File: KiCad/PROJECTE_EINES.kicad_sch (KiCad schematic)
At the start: 5 parts

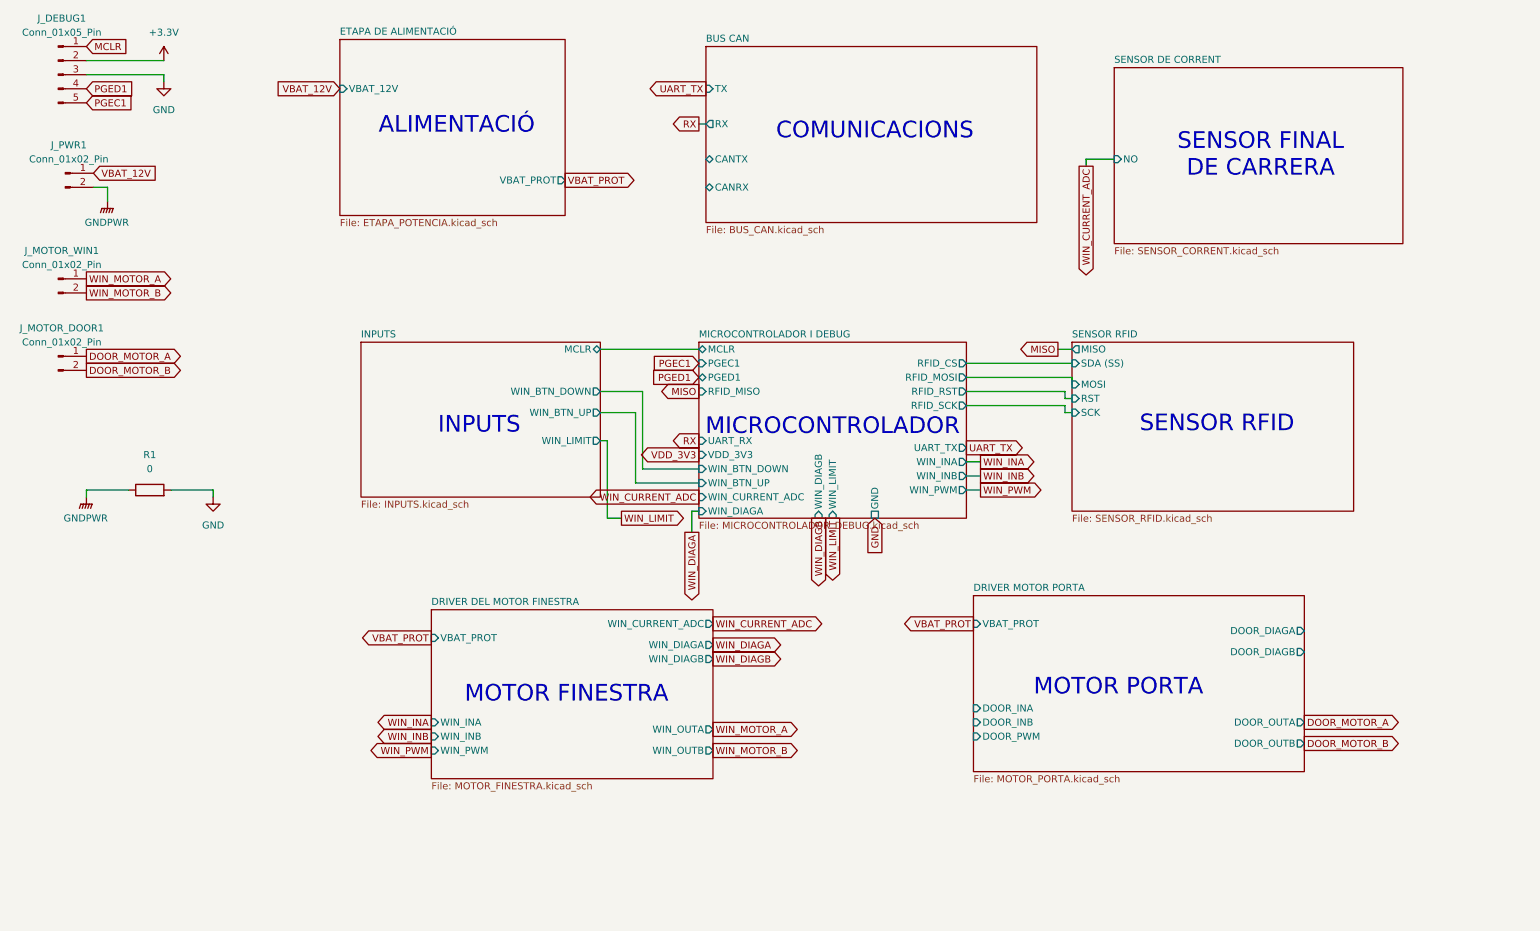
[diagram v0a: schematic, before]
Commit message: Versió final Esquematic
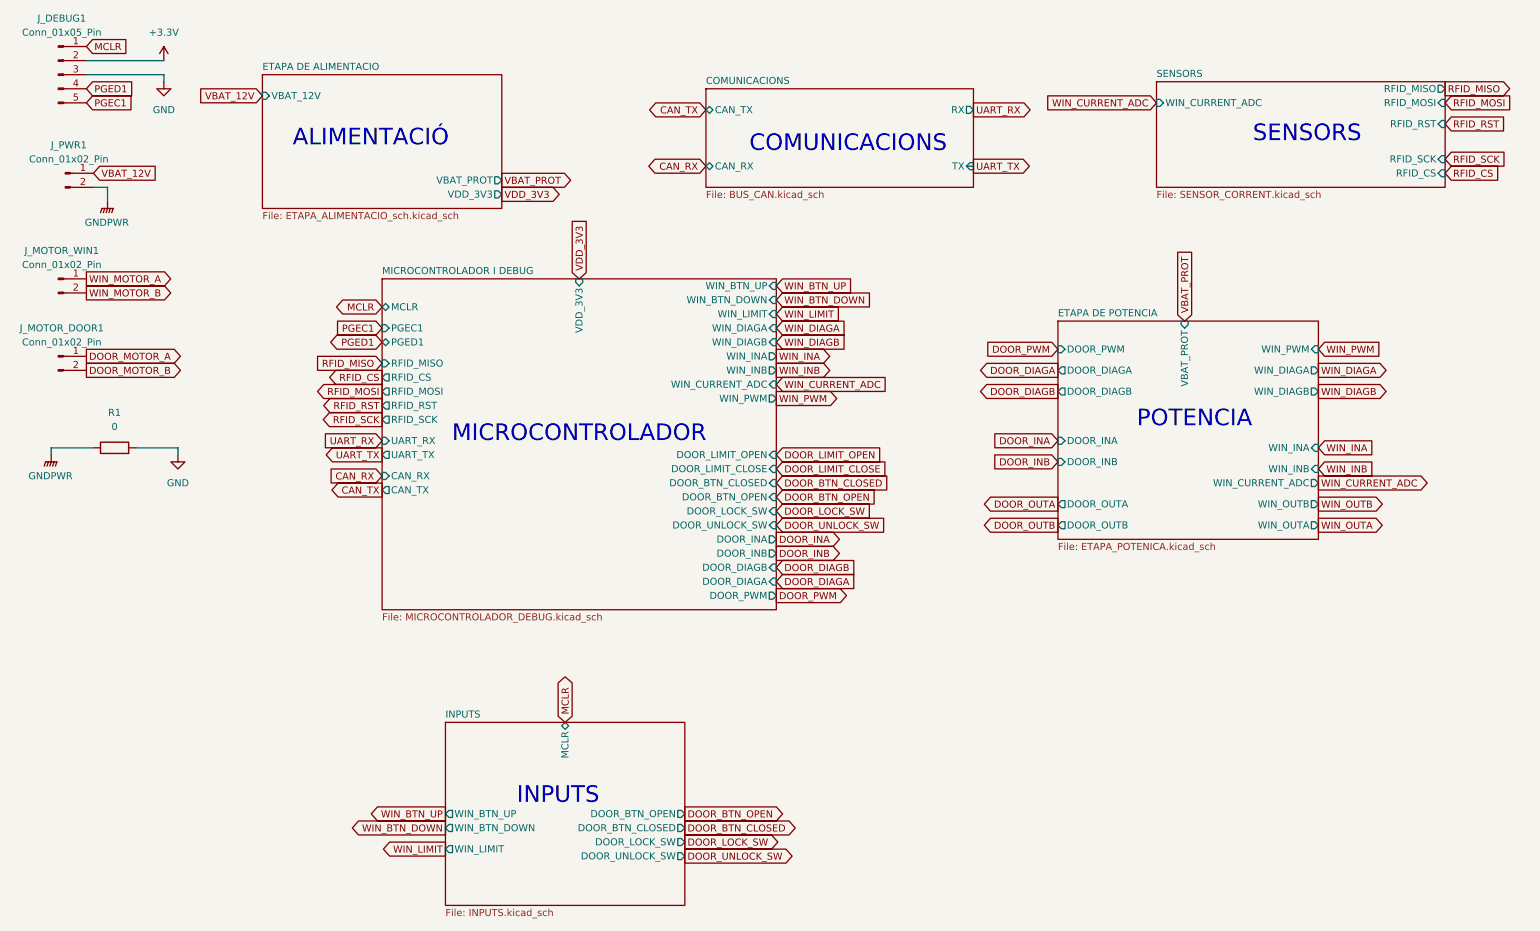
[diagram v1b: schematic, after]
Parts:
- R1: footprint (none) -> Resistor_SMD:R_0805_2012Metric
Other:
- sheet BUS CAN renamed COMUNICACIONS
- sheet SENSOR DE CORRENT renamed SENSORS
- removed sheet DRIVER DEL MOTOR FINESTRA
- removed sheet DRIVER MOTOR PORTA
- removed sheet ETAPA DE ALIMENTACIÓ
- removed sheet SENSOR RFID
- added sheet ETAPA DE ALIMENTACIO (ETAPA_ALIMENTACIO_sch.kicad_sch)
- added sheet ETAPA DE POTENCIA (ETAPA_POTENICA.kicad_sch)
- sheet COMUNICACIONS ports: added CAN_RX, CAN_TX; removed CANRX, CANTX
- sheet INPUTS ports: added DOOR_BTN_CLOSED, DOOR_BTN_OPEN, DOOR_LOCK_SW, DOOR_UNLOCK_SW; removed none
- sheet MICROCONTROLADOR I DEBUG ports: added CAN_RX, CAN_TX, DOOR_BTN_CLOSED, DOOR_BTN_OPEN, DOOR_DIAGA, DOOR_DIAGB, DOOR_INA, DOOR_INB, DOOR_LIMIT_CLOSE, DOOR_LIMIT_OPEN, DOOR_LOCK_SW, DOOR_PWM, DOOR_UNLOCK_SW; removed GND
- sheet SENSORS ports: added RFID_CS, RFID_MISO, RFID_MOSI, RFID_RST, RFID_SCK, WIN_CURRENT_ADC; removed NO
- note added: "POTENCIA"
- note added: "SENSORS"
- note removed: "MOTOR FINESTRA"
- note removed: "MOTOR PORTA"
- note removed: "SENSOR FINAL DE CARRERA"
- note removed: "SENSOR RFID"
- moved on the sheet: R1

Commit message: Versió final de l'esquematic
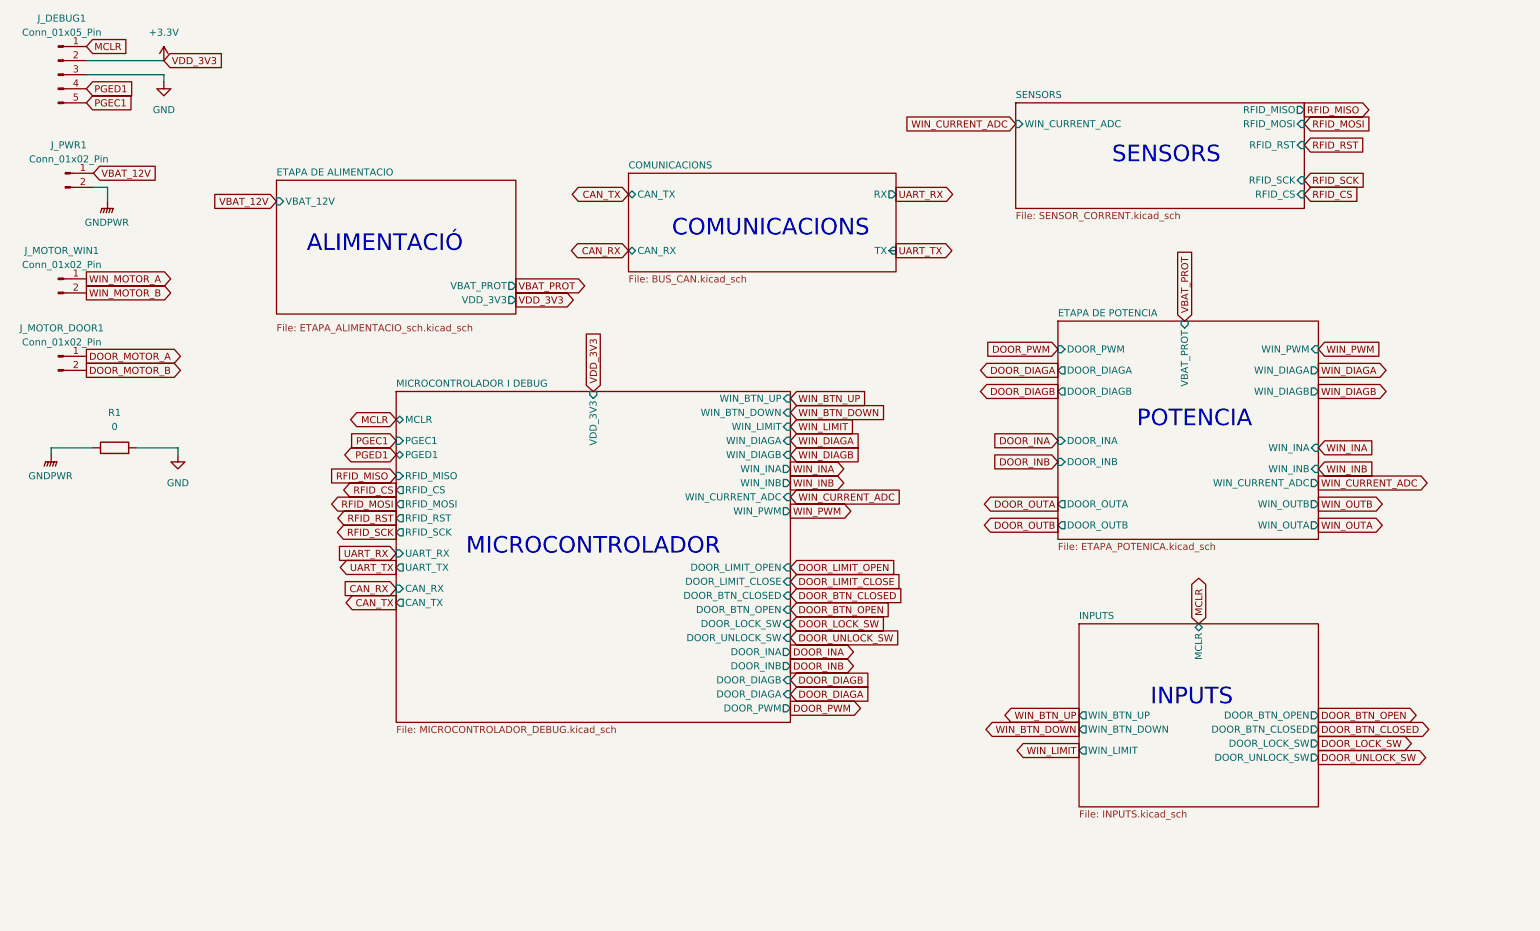
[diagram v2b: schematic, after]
